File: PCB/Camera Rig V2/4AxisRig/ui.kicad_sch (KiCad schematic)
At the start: 3 parts, among them J1 Conn_01x04_Socket, SW3 RotaryEncoder_Switch

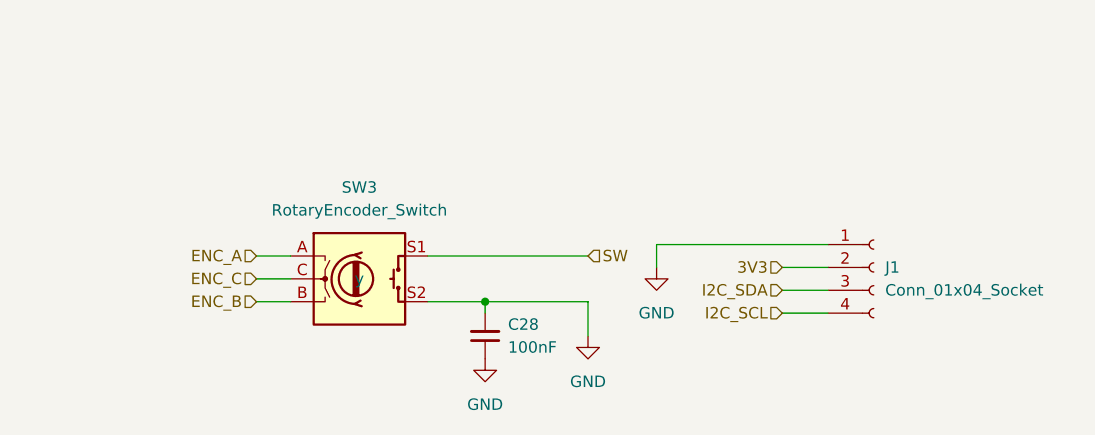
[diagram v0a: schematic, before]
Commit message: PCB V2 first draft
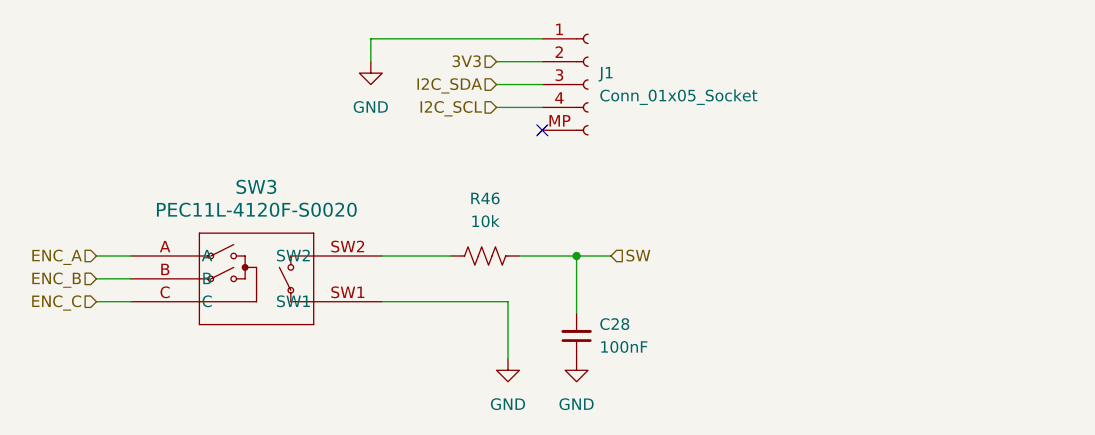
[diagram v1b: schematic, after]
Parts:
- removed J1: Conn_01x04_Socket, Connector_JST:JST_SH_BM04B-SRSS-TB_1x04-1MP_P1.00mm_Vertical, symbol Connector:Conn_01x04_Socket
- removed SW3: RotaryEncoder_Switch, symbol Device:RotaryEncoder_Switch
- added J1: Conn_01x05_Socket, Connector_JST:JST_SH_BM04B-SRSS-TB_1x04-1MP_P1.00mm_Vertical, symbol Connector:Conn_01x05_Socket
- added R46: 10k, Resistor_SMD:R_0603_1608Metric_Pad0.98x0.95mm_HandSolder, symbol Device:R_US
- added SW3: PEC11L-4120F-S0020, PEC11L-4120F-S0020:PEC11L-4x20F-Sxxx_BRN, symbol PEC11L-4120F-S0020:PEC11L-4120F-S0020
- C28: footprint (none) -> Capacitor_SMD:C_0603_1608Metric_Pad1.08x0.95mm_HandSolder
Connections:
- net 3V3: now also J1.2 (Pin_2)
- net ENC_A: now also SW3.A
- net ENC_B: now also SW3.B
- net ENC_C: now also SW3.C
- net GND: now also J1.1 (Pin_1), SW3.SW1; no longer C28.2
- net I2C_SCL: now also J1.4 (Pin_4)
- net I2C_SDA: now also J1.3 (Pin_3)
- net SW: now also C28.2, R46.1
- new net: R46.2, SW3.SW2
- no-connect marks 0 -> 1
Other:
- moved on the sheet: C28
